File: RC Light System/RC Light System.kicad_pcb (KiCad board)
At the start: 2 copper layers, 41.3 x 54 mm, 41 parts, among them J1 INPUT, J10 EX_B, J2 CHAIN, J3 FL_A, J4 FL_B, J5 BR_A, J6 BR_B, J7 BL_L, J8 BL_R, J9 EX_A, Q1 2N2222, Q2 2N2222, Q3 2N2222, Q4 2N2222, Q5 2N2222, Q6 2N2222, Q7 2N2222, Q8 2N2222, U1 74HC595

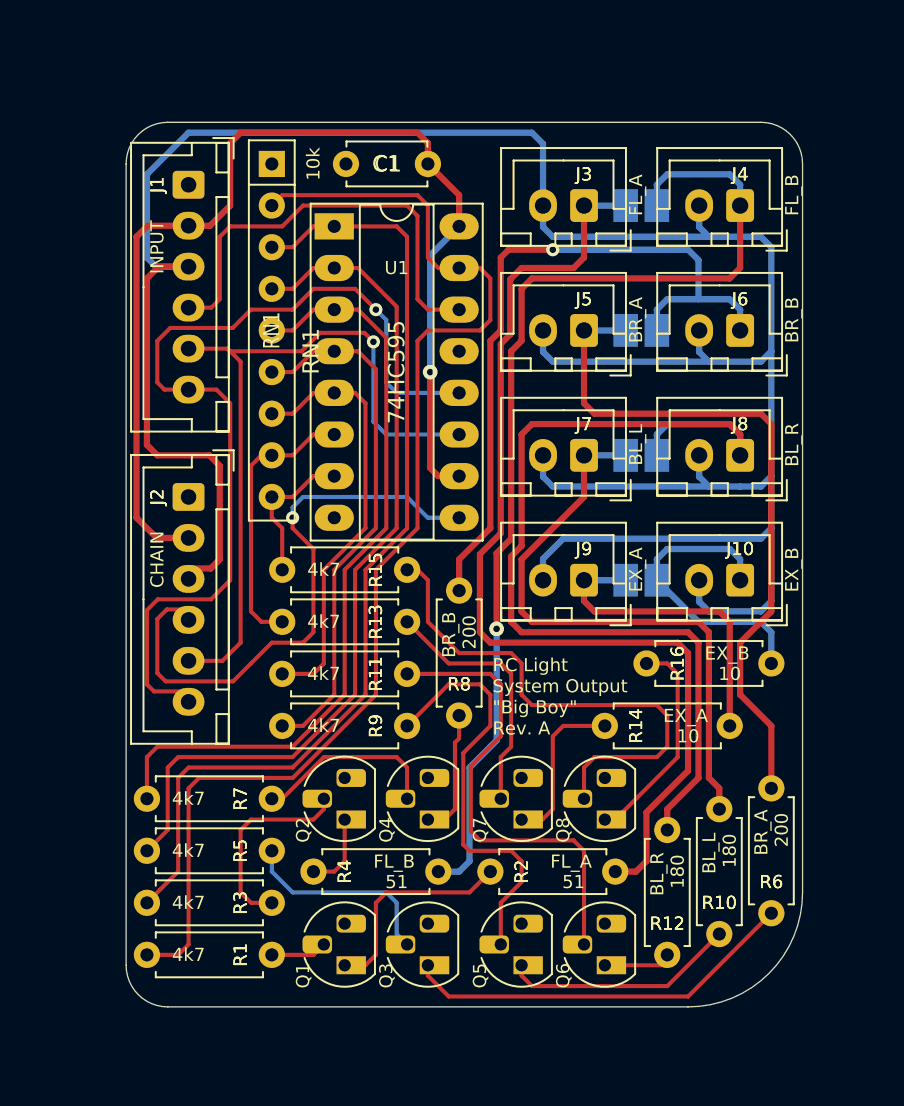
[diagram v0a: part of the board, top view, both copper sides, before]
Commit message: First layout done
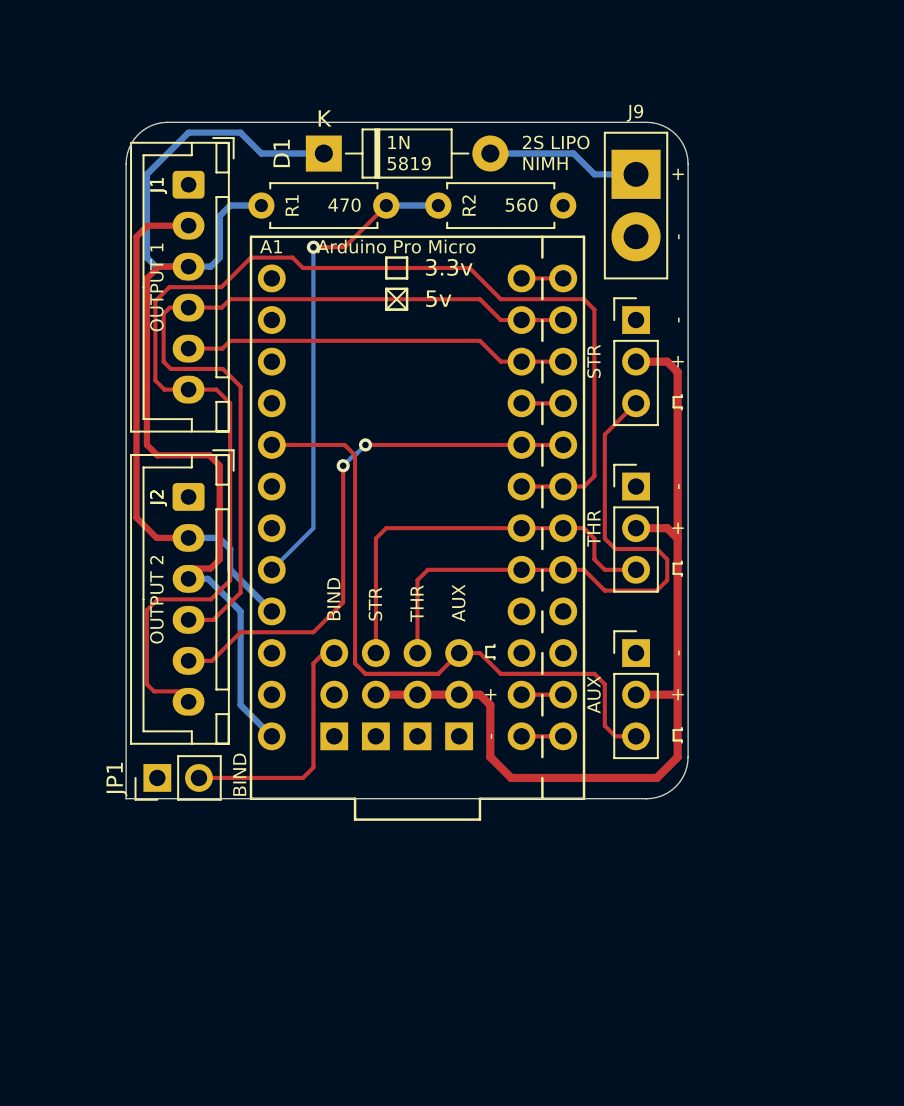
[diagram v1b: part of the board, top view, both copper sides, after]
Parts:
- removed C1: 100nF, Capacitor_THT:C_Disc_D4.7mm_W2.5mm_P5.00mm
- removed JP2: BR_LINK, solder_bridge:bridge_open
- removed JP3: BL_LINK, solder_bridge:bridge_open
- removed JP4: EX_LINK, solder_bridge:bridge_open
- removed Q1, Q2, Q3, Q4, Q5, Q6, Q7, Q8: 2N2222, Package_TO_SOT_THT:TO-92_HandSolder
- removed R10, R12: 180, resistor:R_Axial_DIN0207_L6.3mm_D2.5mm_P7.62mm_Horizontal
- removed R11, R13, R15, R3, R5, R7, R9: 4k7, resistor:R_Axial_DIN0207_L6.3mm_D2.5mm_P7.62mm_Horizontal
- removed R14, R16: 10, resistor:R_Axial_DIN0207_L6.3mm_D2.5mm_P7.62mm_Horizontal
- removed R4: 51, resistor:R_Axial_DIN0207_L6.3mm_D2.5mm_P7.62mm_Horizontal
- removed R6, R8: 200, resistor:R_Axial_DIN0207_L6.3mm_D2.5mm_P7.62mm_Horizontal
- removed RN1: 10k, Resistor_THT:R_Array_SIP9
- removed U1: 74HC595, Package_DIP:DIP-16_W7.62mm_Socket_LongPads
- added A1: Arduino Pro Micro, arduino_pro_micro:Arduino_Pro_Micro, F.Cu at (81.3, 104.8)
- added D1: 1N5819, Diode_THT:D_DO-41_SOD81_P10.16mm_Horizontal, F.Cu at (75.6, 83.2)
- J1: value INPUT -> OUTPUT 1
- J10: value EX_B -> BIND_IN; footprint Connector_JST:JST_XH_B2B-XH-A_1x02_P2.50mm_Vertical -> Connector_PinSocket_2.54mm:PinSocket_1x03_P2.54mm_Vertical; moved to B.Cu
- J2: value CHAIN -> OUTPUT 2
- J3: value FL_A -> STR_IN; footprint Connector_JST:JST_XH_B2B-XH-A_1x02_P2.50mm_Vertical -> Connector_PinSocket_2.54mm:PinSocket_1x03_P2.54mm_Vertical; moved to B.Cu
- J4: value FL_B -> STR_OUT; footprint Connector_JST:JST_XH_B2B-XH-A_1x02_P2.50mm_Vertical -> Connector_PinHeader_2.54mm:PinHeader_1x03_P2.54mm_Vertical
- J5: value BR_A -> THR_IN; footprint Connector_JST:JST_XH_B2B-XH-A_1x02_P2.50mm_Vertical -> Connector_PinSocket_2.54mm:PinSocket_1x03_P2.54mm_Vertical; moved to B.Cu
- J6: value BR_B -> THR_OUT; footprint Connector_JST:JST_XH_B2B-XH-A_1x02_P2.50mm_Vertical -> Connector_PinHeader_2.54mm:PinHeader_1x03_P2.54mm_Vertical
- J7: value BL_L -> AUX_IN; footprint Connector_JST:JST_XH_B2B-XH-A_1x02_P2.50mm_Vertical -> Connector_PinSocket_2.54mm:PinSocket_1x03_P2.54mm_Vertical; moved to B.Cu
- J8: value BL_R -> AUX_OUT; footprint Connector_JST:JST_XH_B2B-XH-A_1x02_P2.50mm_Vertical -> Connector_PinHeader_2.54mm:PinHeader_1x03_P2.54mm_Vertical
- J9: value EX_A -> VBATT; footprint Connector_JST:JST_XH_B2B-XH-A_1x02_P2.50mm_Vertical -> rc_light_system:Conn_Light_Power
- JP1: value FL_LINK -> BIND; footprint solder_bridge:bridge_open -> Connector_PinHeader_2.54mm:PinHeader_1x02_P2.54mm_Vertical; moved to F.Cu
- R1: value 4k7 -> 470
- R2: value 51 -> 560
- moved JP1 46.4 mm to (65.4, 121.3)
- moved R1 45.7 mm to (71.8, 86.4), turned to 0 degrees
- moved R2 40.8 mm to (82.5, 86.4)
- moved J3 33.9 mm to (81.3, 118.7), turned to 0 degrees
- moved J5 27.8 mm to (78.7, 118.7), turned to 0 degrees
- moved J10 26.5 mm to (76.2, 118.7), turned to 0 degrees
- moved J9 25.0 mm to (94.6, 84.5), turned to 90 degrees
- moved J7 18.8 mm to (83.8, 118.7), turned to 0 degrees
- moved J8 13.6 mm to (94.6, 113.7), turned to 0 degrees
- moved J6 11.4 mm to (94.6, 103.5), turned to 0 degrees
- moved J4 9.44 mm to (94.6, 93.3), turned to 0 degrees
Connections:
- J1 pad 5: /SER_CLK -> /SER_CLK_1
- J10 pad 1: Net-(J10-Pad1) -> GND
- J10 pad 2: VCC -> (no net)
- J2 pad 4: Net-(J2-Pad4) -> /SER_DATA
- J2 pad 5: /SER_CLK -> /SER_CLK_2
- J3 pad 1: Net-(J3-Pad1) -> GND
- J3 pad 2: VCC -> /BEC
- J4 pad 1: Net-(J4-Pad1) -> GND
- J4 pad 2: VCC -> /BEC
- J5 pad 1: Net-(J5-Pad1) -> GND
- J5 pad 2: VCC -> /BEC
- J6 pad 1: Net-(J6-Pad1) -> GND
- J6 pad 2: VCC -> /BEC
- J7 pad 1: Net-(J7-Pad1) -> GND
- J7 pad 2: VCC -> /BEC
- J8 pad 1: Net-(J8-Pad1) -> GND
- J8 pad 2: VCC -> /BEC
- J9 pad 2: VCC -> GND
- JP1 pad 1: Net-(J4-Pad1) -> GND
- JP1 pad 2: Net-(J3-Pad1) -> Net-(J10-Pad3)
- R1 pad 1: Net-(Q1-Pad2) -> VCC
- R1 pad 2: FL_A -> Net-(A1-Pad20)
- R2 pad 1: Net-(Q1-Pad1) -> Net-(A1-Pad20)
- R2 pad 2: Net-(J3-Pad1) -> GND
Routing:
- net VCC: track 160.5 -> 65.9 mm
- net FL_A: track 73.8 -> 0.00 mm
- net Net-(J4-Pad1): track 64.2 -> 0.00 mm, vias 1 -> 0
- net Net-(J3-Pad1): track 62.2 -> 0.00 mm
- net FL_B: track 60.0 -> 0.00 mm
- net Net-(J8-Pad1): track 59.1 -> 0.00 mm
- net /BEC: track 0.00 -> 54.5 mm
- net BR_A: track 52.7 -> 0.00 mm
- net BR_B: track 47.2 -> 0.00 mm
- net Net-(J6-Pad1): track 44.4 -> 0.00 mm, vias 1 -> 0
- net /SER_CLK: track 44.1 -> 0.00 mm, vias 1 -> 0
- net Net-(J5-Pad1): track 42.7 -> 0.00 mm
- net /AUX: track 0.00 -> 39.6 mm
- net Net-(J7-Pad1): track 36.7 -> 0.00 mm
- net +5V: track 67.7 -> 32.0 mm, vias 1 -> 0
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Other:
- board size 41.3 x 54 mm -> 34.3 x 41.3 mm
- net class BEC added: clearance 0.2, trace_width 0.5, via_dia 0.8, via_drill 0.4
- board text added: "+"
- board text added: "-"
- board text added: "1N 5819"
- board text added: "2S LIPO NIMH"
- board text added: "AUX"
- board text added: "BIND"
- board text added: "OUTPUT 1"
- board text added: "OUTPUT 2"
- board text added: "RC Light System "Big Chief" Rev. A"
- board text added: "STR"
- board text added: "THR"
- board text removed: "BL_L"
- board text removed: "BL_R"
- board text removed: "BR_A"
- board text removed: "BR_B"
- board text removed: "EX_A"
- board text removed: "EX_B"
- board text removed: "FL_A"
- board text removed: "FL_B"
- board text removed: "RC Light System Output "Big Boy" Rev. A"
